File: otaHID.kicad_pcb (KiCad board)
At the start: 2 copper layers, 14 x 35 mm, 25 parts, among them J1 USB_A, J2 A1001WR-S-2P, J3 STM32_Debug, SW1 TVAF06-A020B-R, U1 NJW4183U3, U2 LXES11DAA2-135, U3 STM32L4P5CGT6, U4 RN4020, U5 TLP172AM, Y1 12MHz

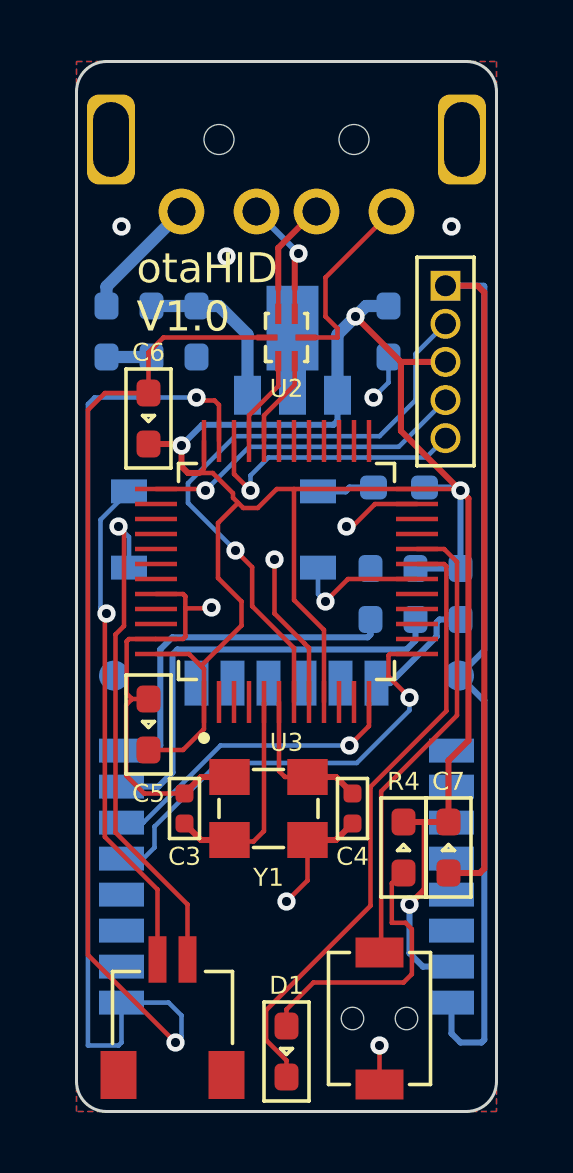
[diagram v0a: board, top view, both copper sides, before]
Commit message: 基盤v2.0
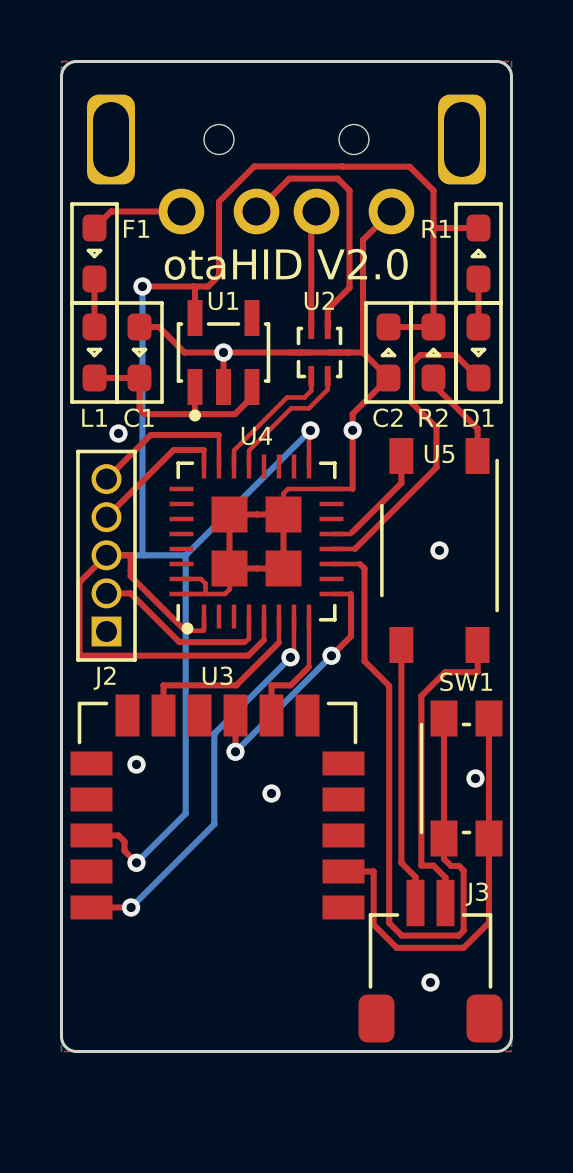
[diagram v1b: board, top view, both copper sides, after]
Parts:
- removed C3, C4: 10pF, otaHID:1005Metric
- removed C5, C6, C7: 0.1uF, otaHID:1608Metric
- removed R3: 10k, otaHID:1608Metric
- removed R4: 1k, otaHID:1608Metric
- removed R5: 470, otaHID:1608Metric
- removed Y1: 12MHz, otaHID:Crystal_SMD_3225-4Pin_3.2x2.5mm_HandSoldering
- C1, F1, L1, U5: moved to F.Cu
- C2: value 2.2uF -> 1uF; moved to F.Cu
- J2: value A1001WR-S-2P -> STM32_Debug; footprint otaHID:A1001WR-S-2P -> otaHID:STM32_Debug_5pin
- J3: value STM32_Debug -> A1001WR-S-2P; footprint otaHID:STM32_Debug_5pin -> otaHID:A1001WR-S-2P
- R1: value 10k -> 1k; moved to F.Cu
- R2: value 10k -> 470; moved to F.Cu
- SW1: footprint otaHID:SW_TVAF06 -> otaHID:SideSW_THAF01-NC-R
- U1: value NJW4183U3 -> NJM12877F33; footprint otaHID:SOT-89-3 -> otaHID:SOT-23-5; moved to F.Cu
- U3: value STM32L4P5CGT6 -> BM71; footprint otaHID:LQFP-48_7x7mm_P0.5mm_FusionPCB -> otaHID:BM71
- U4: value RN4020 -> STM32L412KBTx; footprint otaHID:RN4020 -> otaHID:QFN-32-1EP_5x5mm_P0.5mm_EP3.3x3.3mm; moved to F.Cu
- moved D1 24.2 mm to (6.40, 4.70)
- moved J3 21.0 mm to (4.80, 23.4)
- moved U3 16.2 mm to (-2.30, 28.0), turned to 180 degrees
- moved J2 11.5 mm to (-6.00, 14.0), turned to 180 degrees
- moved R1 11.5 mm to (6.40, 1.40)
- moved SW1 8.51 mm to (6.00, 18.9)
- moved R2 8.32 mm to (4.90, 4.70), turned to -90 degrees
- moved U5 7.23 mm to (5.10, 11.3), turned to -90 degrees
- moved U4 6.52 mm to (-1.00, 11.0), turned to 90 degrees
- moved F1 2.63 mm to (-6.40, 1.40)
- moved U1 2.31 mm to (-2.10, 4.70)
- moved C1 2.02 mm to (-4.90, 4.70), turned to 90 degrees
- moved L1 2.02 mm to (-6.40, 4.70), turned to 90 degrees
- moved U2 1.21 mm to (1.10, 4.70)
- moved C2 0.70 mm to (3.40, 4.70)
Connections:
- C2 pad 1: +3V3 -> +3.3V
- J2 pad 1: Net-(J2-Pad1) -> GND
- J2 pad 2: Net-(J2-Pad2) -> NRST
- J3 pad 1: GND -> Net-(U5-Pad4)
- J3 pad 2: NRST -> Net-(J3-Pad2)
- R1 pad 1: +3V3 -> +3.3V
- R1 pad 2: Net-(R1-Pad2) -> Net-(D1-Pad2)
- R2 pad 1: Net-(R2-Pad1) -> +3.3V
- R2 pad 2: GND -> Net-(R2-Pad2)
- SW1 pad 1: GND -> USER_SW
- SW1 pad 2: USER_SW -> GND
- U1 pad 1: +3V3 -> +5V
- U3 pad 1: +3V3 -> unconnected-(U3-Pad1)
- U3 pad 10: unconnected-(U3-Pad10) -> BM71_RESET
- U3 pad 12: USART2_TX -> unconnected-(U3-Pad12)
- U3 pad 13: USART2_RX -> GND
- U3 pad 14: unconnected-(U3-Pad14) -> +3.3V
- U3 pad 16: unconnected-(U3-Pad16) -> BM71_CONFIG
- U3 pad 2: unconnected-(U3-Pad2) -> GND
- U3 pad 5: OSC_I -> unconnected-(U3-Pad5)
- U3 pad 6: OSC_O -> unconnected-(U3-Pad6)
- U3 pad 7: NRST -> USART2_TX
- U3 pad 8: GND -> USART2_RX
- U3 pad 9: +3V3 -> unconnected-(U3-Pad9)
- U4 pad 1: GND -> +3.3V
- U4 pad 11: unconnected-(U4-Pad11) -> USER_SW
- U4 pad 12: unconnected-(U4-Pad12) -> STATUS_LED
- U4 pad 13: unconnected-(U4-Pad13) -> POWER_SW
- U4 pad 15: Net-(R3-Pad2) -> unconnected-(U4-Pad15)
- U4 pad 17: unconnected-(U4-Pad17) -> +3.3V
- U4 pad 21: unconnected-(U4-Pad21) -> USB_DM
- U4 pad 22: unconnected-(U4-Pad22) -> USB_DP
- U4 pad 23: +3V3 -> SWDIO
- U4 pad 24: GND -> SWCLK
- U4 pad 4: unconnected-(U4-Pad4) -> NRST
- U4 pad 5: USART2_RX -> +3.3V
- U4 pad 6: USART2_TX -> BM71_RESET
- U4 pad 7: Net-(R1-Pad2) -> BM71_CONFIG
- U4 pad 8: Net-(R2-Pad1) -> USART2_TX
- U4 pad 9: GND -> USART2_RX
- U5 pad 1: Net-(R5-Pad2) -> Net-(R2-Pad2)
- U5 pad 4: Net-(J2-Pad2) -> Net-(U5-Pad4)
- U5 pad 6: Net-(J2-Pad1) -> Net-(J3-Pad2)
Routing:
- net GND: track 149.4 -> 47.4 mm, vias 11 -> 8
- net +3V3: track 77.0 -> 0.00 mm, vias 4 -> 0
- net +3.3V: track 0.00 -> 69.5 mm, vias 0 -> 3
- net Net-(J2-Pad2): track 17.1 -> 0.00 mm, vias 1 -> 0
- net Net-(J2-Pad1): track 16.8 -> 0.00 mm, vias 1 -> 0
- net Net-(R1-Pad2): track 14.8 -> 0.00 mm
- net NRST: track 20.4 -> 6.16 mm, vias 1 -> 0
- net BM71_CONFIG: track 0.00 -> 13.3 mm, vias 0 -> 2
- net Net-(R2-Pad1): track 12.3 -> 0.00 mm
- net Net-(J3-Pad2): track 0.00 -> 10.6 mm
- net STATUS_LED: track 20.8 -> 11.1 mm
- net Net-(U5-Pad4): track 0.00 -> 8.79 mm
- net USER_SW: track 15.6 -> 23.5 mm
- net Net-(D1-Pad2): track 9.32 -> 1.60 mm
- net OSC_I: track 7.34 -> 0.00 mm
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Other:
- board size 14 x 35 mm -> 15 x 33 mm
- board text added: "otaHID V2.0"
- board text removed: "otaHID V1.0"

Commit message: 基板 V2.1
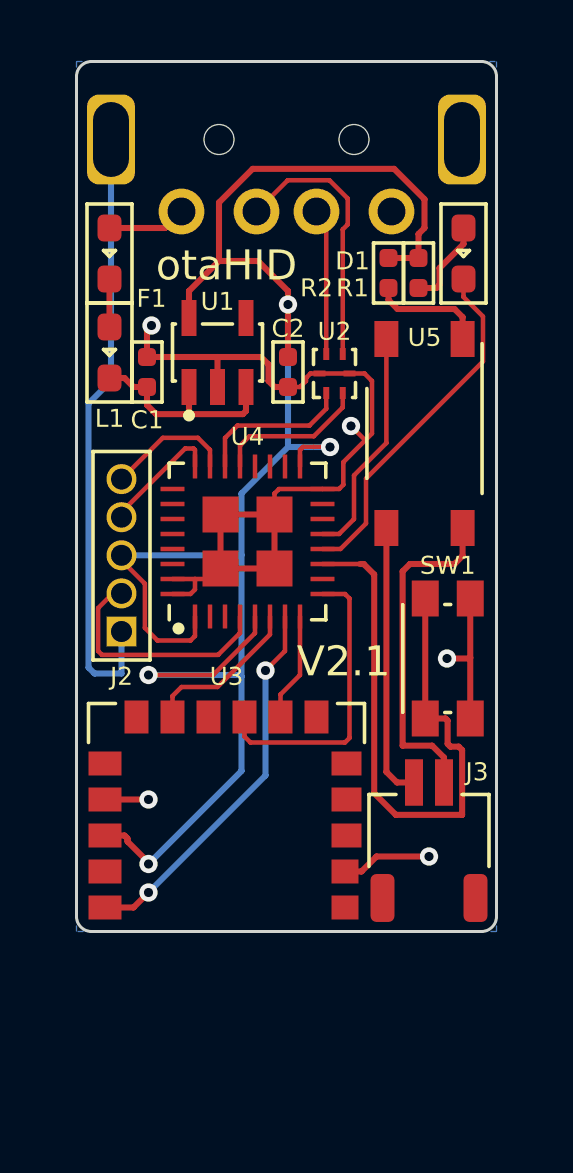
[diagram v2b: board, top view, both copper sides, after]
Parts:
- C1, C2, R1, R2: footprint otaHID:1608Metric -> otaHID:1005Metric
- moved SW1 4.05 mm to (5.38, 14.9)
- moved J3 4.02 mm to (4.75, 19.4)
- moved U5 3.93 mm to (4.60, 7.40)
- moved C2 3.41 mm to (0.05, 5.35)
- moved D1 3.34 mm to (5.90, 1.40)
- moved R2 3.05 mm to (3.40, 2.05)
- moved R1 2.10 mm to (4.40, 2.05)
- moved U2 0.86 mm to (1.60, 5.40)
- moved C1 0.70 mm to (-4.65, 5.35)
- moved F1 0.50 mm to (-5.90, 1.40)
- moved J2 0.50 mm to (-5.50, 14.0)
- moved L1 0.50 mm to (-5.90, 4.70)
- moved U4 0.30 mm to (-1.30, 11.0)
- moved U3 0.30 mm to (-2.00, 28.0)
- moved U1 0.20 mm to (-2.30, 4.70)
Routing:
- net GND: track 47.4 -> 58.2 mm, vias 8 -> 5
- net +3.3V: track 69.5 -> 62.5 mm, vias 3 -> 4
- net POWER_SW: track 3.94 -> 7.71 mm
- net USER_SW: track 23.5 -> 20.7 mm
- net NRST: track 6.16 -> 8.05 mm
- net Net-(D1-Pad2): track 1.60 -> 2.97 mm
- net USART2_RX: track 8.71 -> 9.91 mm, vias 2 -> 0
- net SWDIO: track 5.41 -> 4.24 mm
- net BM71_RESET: track 6.32 -> 5.40 mm
- net /D+: track 3.98 -> 4.88 mm
- net USB_DP: track 4.42 -> 5.25 mm
- net STATUS_LED: track 11.1 -> 11.8 mm
- net Net-(J3-Pad2): track 10.6 -> 11.3 mm
- net +5V: track 7.84 -> 7.15 mm
- net USB_DM: track 4.45 -> 5.13 mm
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- removed copper zone on F.Cu, net GND
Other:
- board size 15 x 33 mm -> 14 x 29 mm
- board text added: "V2.1"
- board text added: "otaHID"
- board text removed: "otaHID V2.0"
